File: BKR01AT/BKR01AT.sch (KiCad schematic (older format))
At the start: 44 parts, among them J1 Conn_02x03_Odd_Even, SW1 SW_Push, SW2 SW_Push, SW3 SW_Push, U1 LIS2DHTR, Y1 32MHz, Y2 32.768kHz

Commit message: WIP: PCB
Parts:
- AE1: footprint antena_ble:2450AT18B100 -> 2450AT18B100E:ANT_2450AT18B100E
- D1, D2, D3: footprint (none) -> LED_SMD:LED_0603_1608Metric
- FID1, FID2: footprint (none) -> Fiducial:Fiducial_0.5mm_Mask1mm
- MCU1: footprint (none) -> Package_DFN_QFN:QFN-48-1EP_6x6mm_P0.4mm_EP4.6x4.6mm
- SW1, SW2, SW3: footprint (none) -> Button_Switch_THT:SW_PUSH_6mm_H4.3mm
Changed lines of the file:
@@
 F 0 "SW1" H 9650 5530 50  0000 C CNN
 F 1 "SW_Push" H 9650 5439 50  0000 C CNN
-F 2 "" H 9650 5445 50  0001 C CNN
+F 2 "Button_Switch_THT:SW_PUSH_6mm_H4.3mm" H 9650 5445 50  0001 C CNN
 F 3 "~" H 9650 5445 50  0001 C CNN
 F 4 "PTS636 SL43 LFS" H 9650 5245 50  0001 C CNN "Part Number"
@@
 F 0 "SW3" H 8880 5550 50  0000 C CNN
 F 1 "SW_Push" H 8880 5459 50  0000 C CNN
-F 2 "" H 8880 5465 50  0001 C CNN
+F 2 "Button_Switch_THT:SW_PUSH_6mm_H4.3mm" H 8880 5465 50  0001 C CNN
 F 3 "~" H 8880 5465 50  0001 C CNN
 F 4 "PTS636 SL43 LFS" H 8880 5265 50  0001 C CNN "Part Number"
@@
 F 0 "SW2" H 8055 5535 50  0000 C CNN
 F 1 "SW_Push" H 8055 5444 50  0000 C CNN
-F 2 "" H 8055 5450 50  0001 C CNN
+F 2 "Button_Switch_THT:SW_PUSH_6mm_H4.3mm" H 8055 5450 50  0001 C CNN
 F 3 "~" H 8055 5450 50  0001 C CNN
 F 4 "PTS636 SL43 LFS" H 8055 5250 50  0001 C CNN "Part Number"
@@
 F 0 "D2" V 8752 3313 50  0000 L CNN
 F 1 "Red LED" V 8843 3313 50  0000 L CNN
-F 2 "" H 8805 3235 50  0001 C CNN
+F 2 "LED_SMD:LED_0603_1608Metric" H 8805 3235 50  0001 C CNN
 F 3 "~" H 8805 3235 50  0001 C CNN
 F 4 "150060VS75000" H 8805 3235 50  0001 C CNN "Part Number"
@@
 F 0 "D3" V 8012 3338 50  0000 L CNN
 F 1 "Red LED" V 8103 3338 50  0000 L CNN
-F 2 "" H 8065 3260 50  0001 C CNN
+F 2 "LED_SMD:LED_0603_1608Metric" H 8065 3260 50  0001 C CNN
 F 3 "~" H 8065 3260 50  0001 C CNN
 F 4 "150060RS75000" H 8065 3260 50  0001 C CNN "Part Number"
@@
 F 0 "D1" V 9562 3298 50  0000 L CNN
 F 1 "Green LED" V 9653 3298 50  0000 L CNN
-F 2 "" H 9615 3220 50  0001 C CNN
+F 2 "LED_SMD:LED_0603_1608Metric" H 9615 3220 50  0001 C CNN
 F 3 "~" H 9615 3220 50  0001 C CNN
 F 4 "150060VS75000" H 9615 3220 50  0001 C CNN "Part Number"
@@
 F 0 "FID2" H 7430 6176 50  0000 L CNN
 F 1 "Fiducial" H 7430 6085 50  0000 L CNN
-F 2 "" H 7345 6130 50  0001 C CNN
+F 2 "Fiducial:Fiducial_0.5mm_Mask1mm" H 7345 6130 50  0001 C CNN
 F 3 "~" H 7345 6130 50  0001 C CNN
 	1    7345 6130
@@
 F 0 "FID1" H 8095 6151 50  0000 L CNN
 F 1 "Fiducial" H 8095 6060 50  0000 L CNN
-F 2 "" H 8010 6105 50  0001 C CNN
+F 2 "Fiducial:Fiducial_0.5mm_Mask1mm" H 8010 6105 50  0001 C CNN
 F 3 "~" H 8010 6105 50  0001 C CNN
 	1    8010 6105
@@
 F 0 "MCU1" H 3600 3390 50  0000 L CNN
 F 1 "nRF52832-QFAB-R" H 3335 3305 50  0000 L CNN
-F 2 "" H 3705 3330 50  0001 C CNN
+F 2 "Package_DFN_QFN:QFN-48-1EP_6x6mm_P0.4mm_EP4.6x4.6mm" H 3705 3330 50  0001 C CNN
 F 3 "" H 3705 3330 50  0001 C CNN
 F 4 "nRF52832-QFAB-R" H 3705 3330 50  0001 C CNN "Part Number"
@@
 F 0 "AE1" H 2425 5684 50  0000 L CNN
 F 1 "Antenna" H 2425 5593 50  0000 L CNN
-F 2 "antena_ble:2450AT18B100" H 2345 5695 50  0001 C CNN
+F 2 "2450AT18B100E:ANT_2450AT18B100E" H 2345 5695 50  0001 C CNN
 F 3 "~" H 2345 5695 50  0001 C CNN
 F 4 "2450AT18B100E" H 2345 5695 50  0001 C CNN "Part Number"
@@
 	3005 6510 3005 7645
 $Comp
-L power:VDD #PWR?
+L power:VDD #PWR0101
 U 1 1 5E5987B3
 P 8065 2790
-F 0 "#PWR?" H 8065 2640 50  0001 C CNN
+F 0 "#PWR0101" H 8065 2640 50  0001 C CNN
 F 1 "VDD" H 8082 2963 50  0000 C CNN
 F 2 "" H 8065 2790 50  0001 C CNN
@@
 $EndComp
 $Comp
-L power:VDD #PWR?
+L power:VDD #PWR0102
 U 1 1 5E59EF9F
 P 8805 2765
-F 0 "#PWR?" H 8805 2615 50  0001 C CNN
+F 0 "#PWR0102" H 8805 2615 50  0001 C CNN
 F 1 "VDD" H 8822 2938 50  0000 C CNN
 F 2 "" H 8805 2765 50  0001 C CNN
@@
 $EndComp
 $Comp
-L power:VDD #PWR?
+L power:VDD #PWR0103
 U 1 1 5E5A4F33
 P 9615 2750
-F 0 "#PWR?" H 9615 2600 50  0001 C CNN
+F 0 "#PWR0103" H 9615 2600 50  0001 C CNN
 F 1 "VDD" H 9632 2923 50  0000 C CNN
 F 2 "" H 9615 2750 50  0001 C CNN
@@
 	8055 4745 8055 4690
 $Comp
-L power:VDD #PWR?
+L power:VDD #PWR0104
 U 1 1 5E5B249E
 P 8055 4690
-F 0 "#PWR?" H 8055 4540 50  0001 C CNN
+F 0 "#PWR0104" H 8055 4540 50  0001 C CNN
 F 1 "VDD" H 8072 4863 50  0000 C CNN
 F 2 "" H 8055 4690 50  0001 C CNN
@@
 $EndComp
 $Comp
-L power:VDD #PWR?
+L power:VDD #PWR0105
 U 1 1 5E5B8527
 P 8880 4705
-F 0 "#PWR?" H 8880 4555 50  0001 C CNN
+F 0 "#PWR0105" H 8880 4555 50  0001 C CNN
 F 1 "VDD" H 8897 4878 50  0000 C CNN
 F 2 "" H 8880 4705 50  0001 C CNN
@@
 $EndComp
 $Comp
-L power:VDD #PWR?
+L power:VDD #PWR0106
 U 1 1 5E5BE646
 P 9650 4685
-F 0 "#PWR?" H 9650 4535 50  0001 C CNN
+F 0 "#PWR0106" H 9650 4535 50  0001 C CNN
 F 1 "VDD" H 9667 4858 50  0000 C CNN
 F 2 "" H 9650 4685 50  0001 C CNN

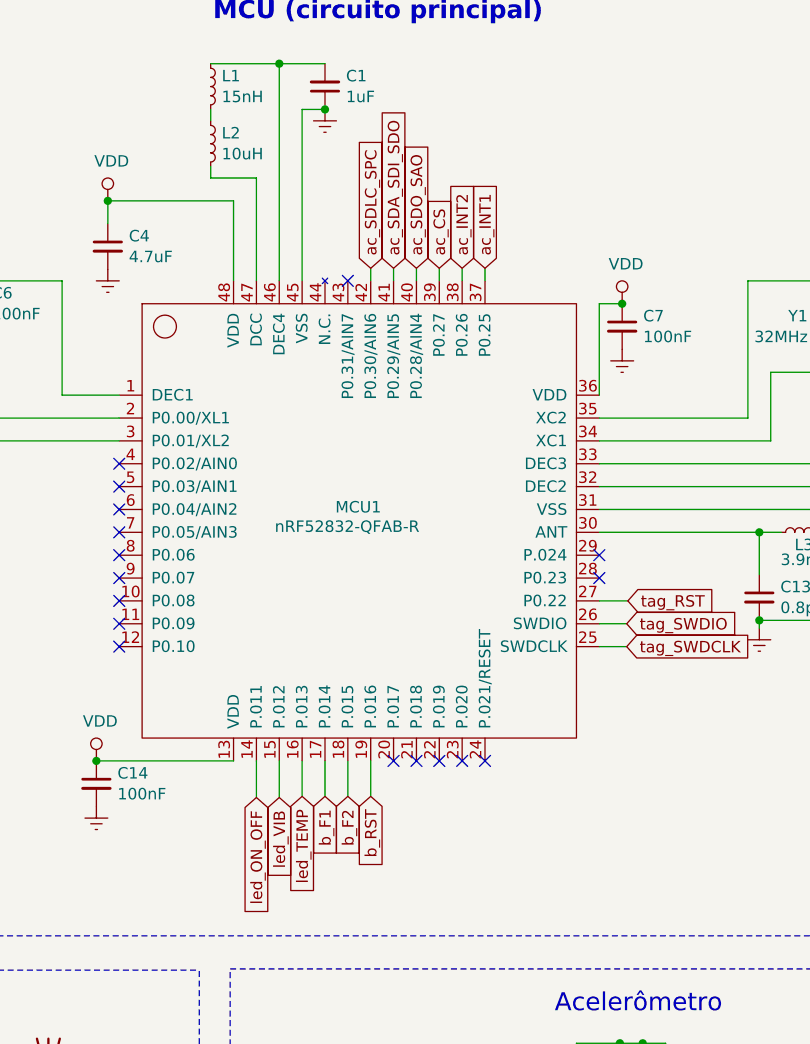
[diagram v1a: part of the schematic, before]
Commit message: PCB: trilhas
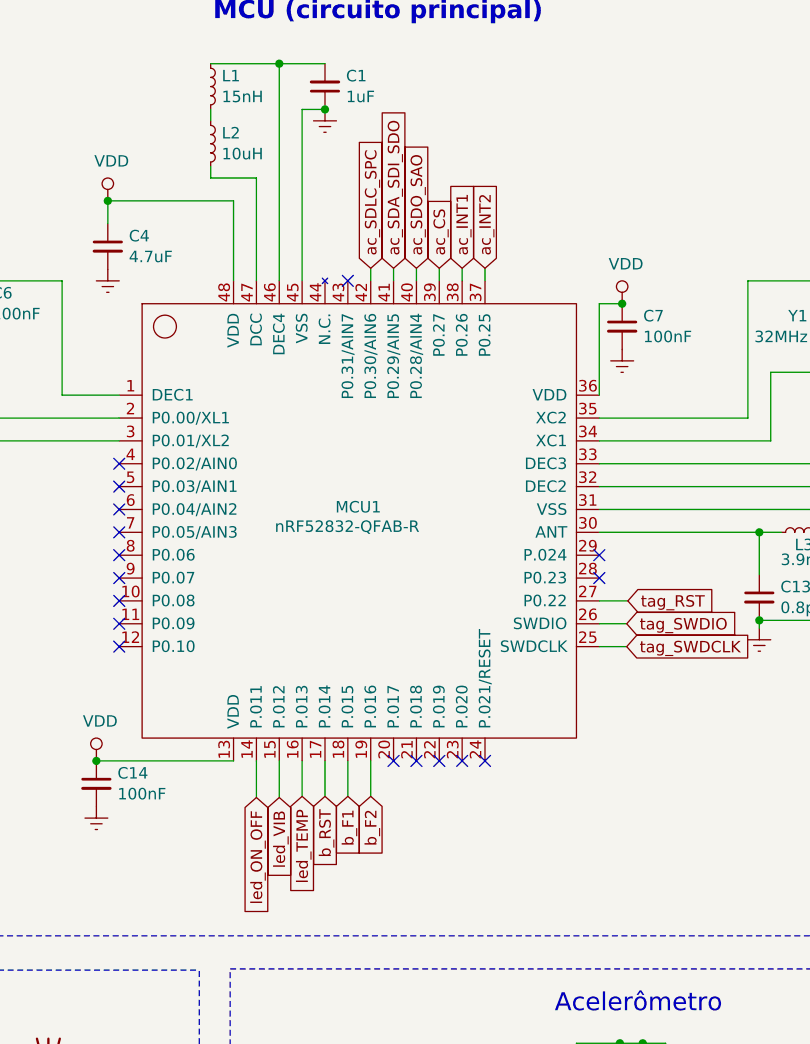
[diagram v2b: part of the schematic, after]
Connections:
- net ac_INT1: now also MCU1.38 (P0.26); no longer MCU1.37 (P0.25)
- net ac_INT2: now also MCU1.37 (P0.25); no longer MCU1.38 (P0.26)
- net b_F1: now also MCU1.18 (P.015); no longer MCU1.17 (P.014)
- net b_F2: now also MCU1.19 (P.016); no longer MCU1.18 (P.015)
- net b_RST: now also MCU1.17 (P.014); no longer MCU1.19 (P.016)
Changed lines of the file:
@@
 Wire Wire Line
 	8055 5040 8055 5050
+Text GLabel 3555 4535 3    50   Input ~ 0
+b_RST
+Text GLabel 3655 4535 3    50   Input ~ 0
+b_F1
 Text GLabel 3755 4535 3    50   Input ~ 0
-b_RST
-Text GLabel 3555 4535 3    50   Input ~ 0
-b_F1
-Text GLabel 3655 4535 3    50   Input ~ 0
 b_F2
 Wire Wire Line
@@
 Wire Wire Line
 	1130 7275 1435 7275
-Text GLabel 4880 3680 2    50   Input ~ 0
-tag_RST
 Text GLabel 4875 3780 2    50   Input ~ 0
 tag_SWDIO
@@
 Text GLabel 3955 2225 1    50   Input ~ 0
 ac_SDO_SAO
+Text GLabel 4255 2225 1    50   Input ~ 0
+ac_INT2
 Text GLabel 4155 2225 1    50   Input ~ 0
-ac_INT2
-Text GLabel 4255 2225 1    50   Input ~ 0
 ac_INT1
 Text GLabel 3855 2225 1    50   Input ~ 0
@@
 NoConn ~ 4055 4380
 NoConn ~ 4155 4380
-NoConn ~ 4255 4380
-Wire Wire Line
-	4880 3680 4755 3680
 $Comp
 L Device:C_Small C13
@@
 $EndComp
 NoConn ~ 5045 6905
+Wire Wire Line
+	4880 3680 4755 3680
+Text GLabel 4880 3680 2    50   Input ~ 0
+tag_RST
+NoConn ~ 4255 4380
 $EndSCHEMATC
